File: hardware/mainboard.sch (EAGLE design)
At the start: 27 parts, among them IC1 ESP-12E/F, Q1 BC847BS, Q2 BC847BS, Q3 BC847BS

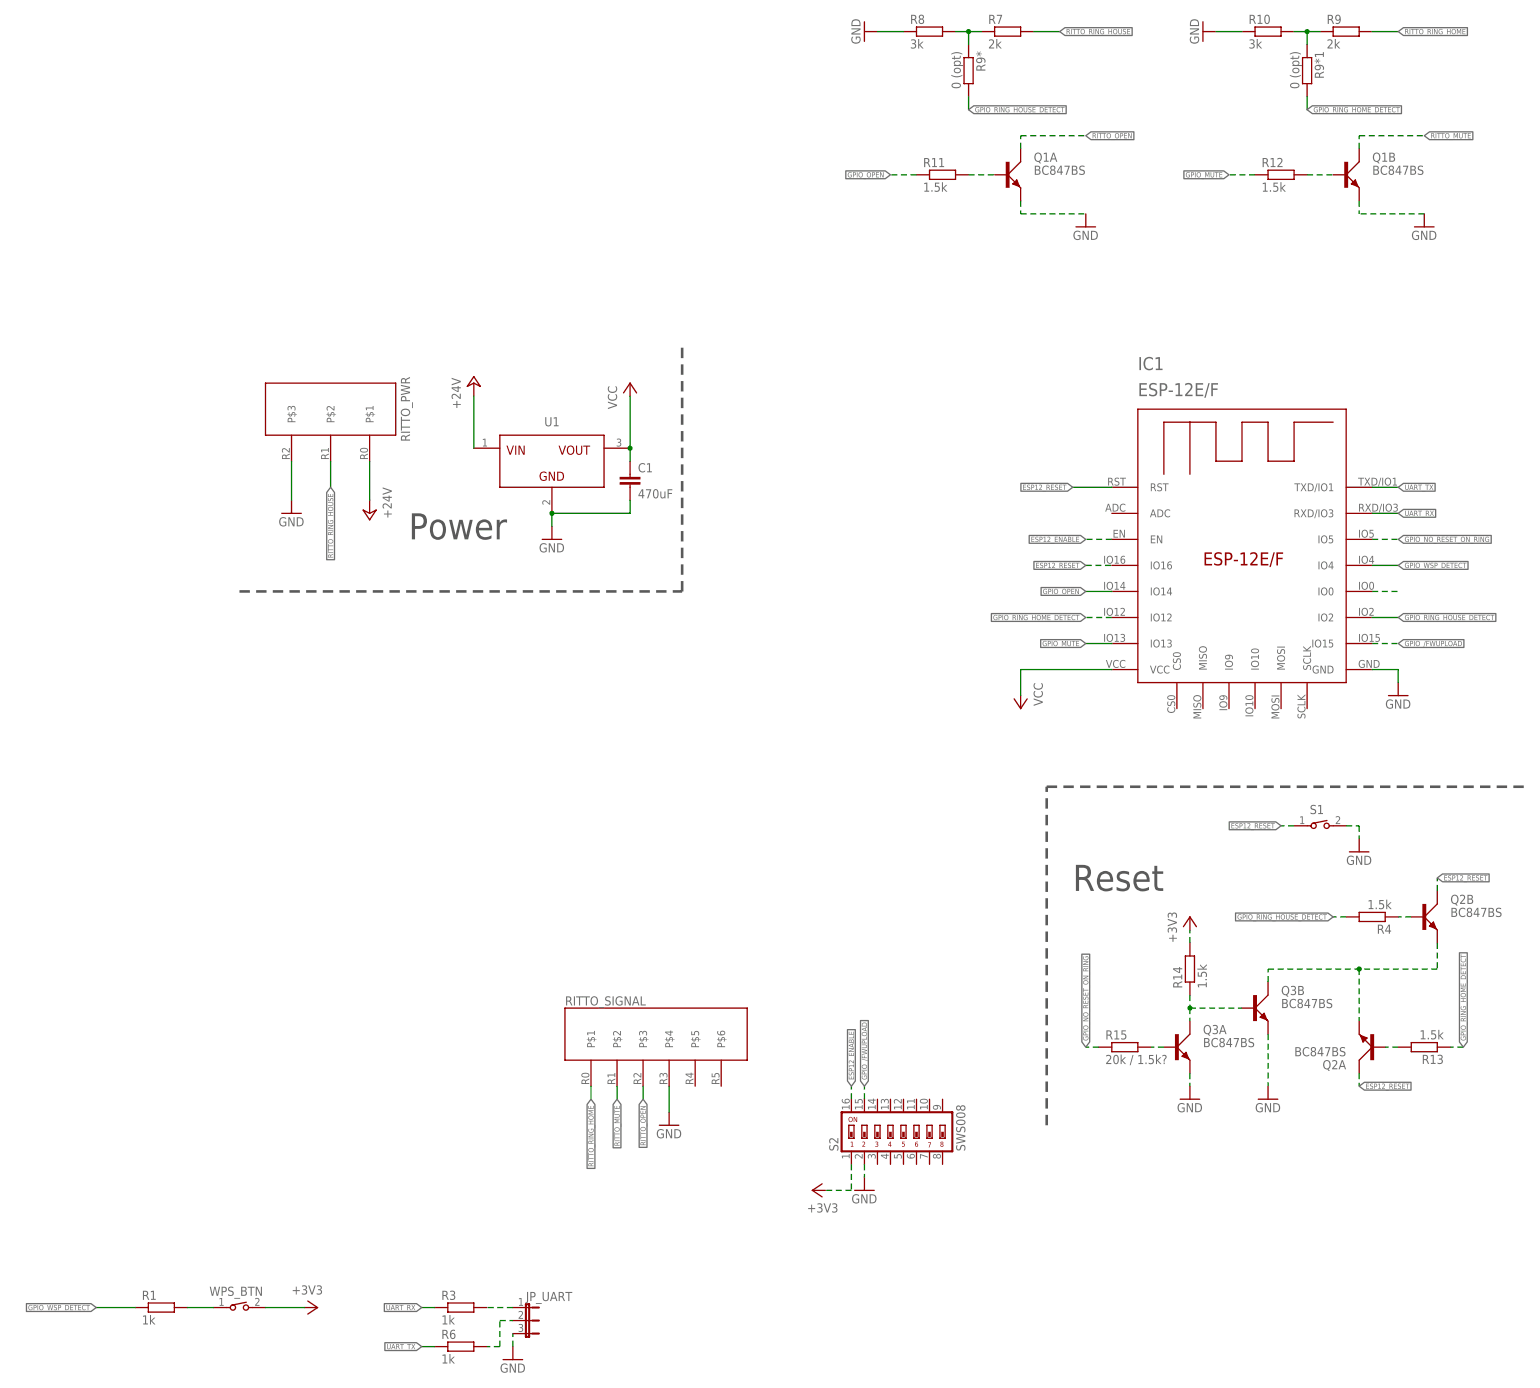
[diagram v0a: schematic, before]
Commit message: Adding latest version of schematic
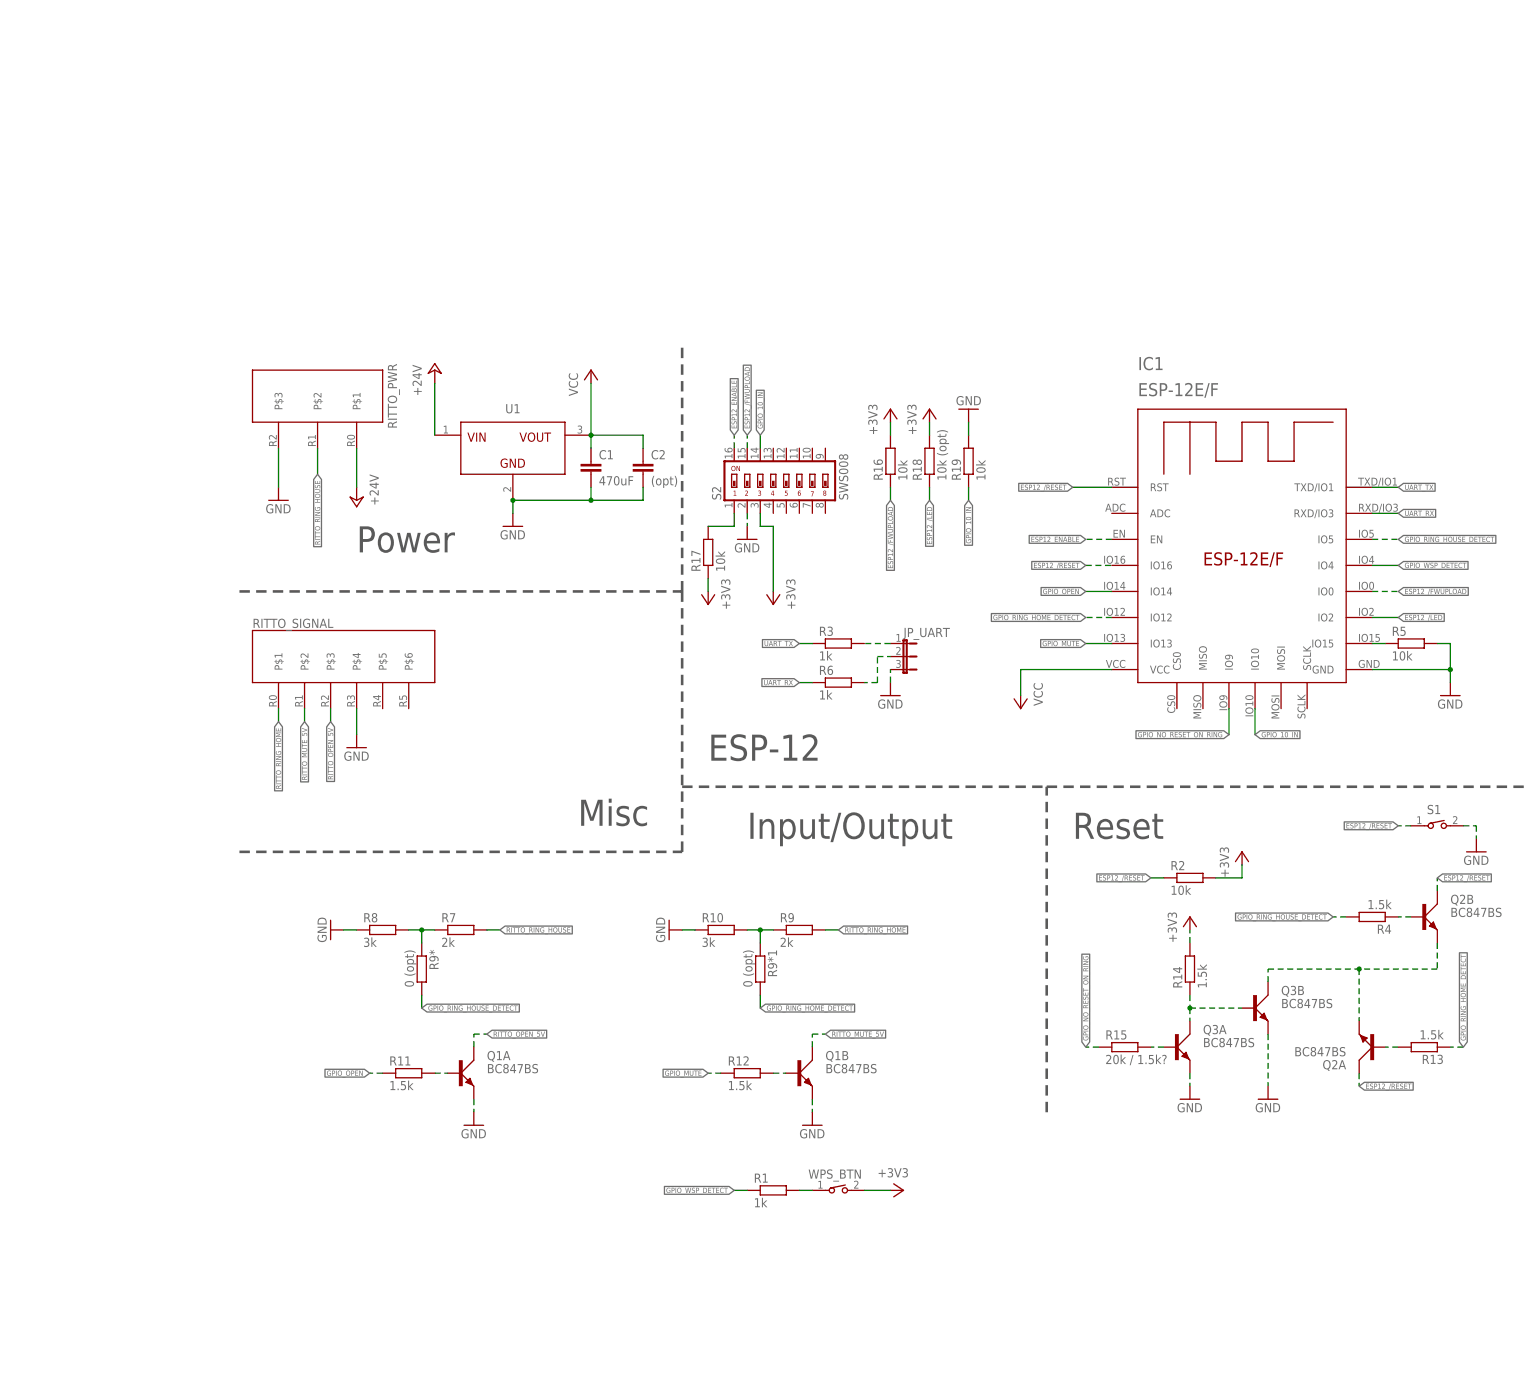
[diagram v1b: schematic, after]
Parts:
- added C2: (opt), rcl:C-EUC1206
- added R16, R17, R19, R2, R5: 10k, rcl:R-EU_R1206
- added R18: 10k (opt), rcl:R-EU_R1206
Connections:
- net RITTO_MUTE renamed RITTO_MUTE_5V
- net RITTO_OPEN renamed RITTO_OPEN_5V
- removed net ESP12_RESET: IC1.IO16, IC1.RST, Q2A.C, Q2B.C, S1.1
- removed net GPIO_/FWUPLOAD: IC1.IO15, S2.15
- new net ESP12_/FWUPLOAD: IC1.IO0, R16.1, S2.15
- new net ESP12_/LED: IC1.IO2, R18.1
- new net ESP12_/RESET: IC1.IO16, IC1.RST, Q2A.C, Q2B.C, R2.1, S1.1
- new net GPIO_10_IN: IC1.IO10, R19.1, S2.14
- new net N$7: R17.2, S2.1
- net +3V3: now also C2.1, R16.2, R17.1, R18.2, R2.2, S2.3; no longer S2.1
- net GND: now also C2.2, R19.2, R5.2
- net GPIO_NO_RESET_ON_RING: now also IC1.IO9; no longer IC1.IO5
- net GPIO_RING_HOUSE_DETECT: now also IC1.IO5; no longer IC1.IO2
- net N$3: now also IC1.IO15, R5.1; no longer IC1.IO0
- net UART_RX: now also R6.1; no longer R3.1
- net UART_TX: now also R3.1; no longer R6.1
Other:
- note added: "ESP-12"
- note added: "Input/Output"
- note added: "Misc"
- moved on the sheet: C1, JP_UART, Q1A, Q1B, R1, R10, R11, R12, R3, R6, R7, R8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
